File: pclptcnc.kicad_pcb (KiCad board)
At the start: 2 copper layers, 180.5 x 52.3 mm, 249 parts, among them P1 ARK825A-3, P3 ARK825A-4, P4 ARK825A-3, P5 ARK825A-3, P6 ARK825A-3, P7 ARK825A-3, P8 ARK825A-3, Q1 BC807-40, Q10 BC807-40, Q11 BC807-40, Q12 BC807-40, Q13 BC807-40, Q14 BC807-40, Q15 BC807-40, Q16 BC807-40, Q17 BC807-40, Q18 BC807-40, Q2 BC807-40, Q3 BC807-40, Q4 BC807-40, Q5 BC807-40, Q6 BC807-40, Q7 BC807-40, Q8 BC807-40, Q9 BC807-40, U1 74LVC1G3157GW, U10 SN74LVC2G17, U11 74HCT14, U12 SN74LVC2G17, U13 74HCT14, U2 HCPL2630, U3 HCPL2630, U4 HCPL2630, U5 HCPL2630, U6 HCPL2630, U7 HCPL2630, U8 74HCT14, U9 74HCT14, j1 DB25, j2 DB25

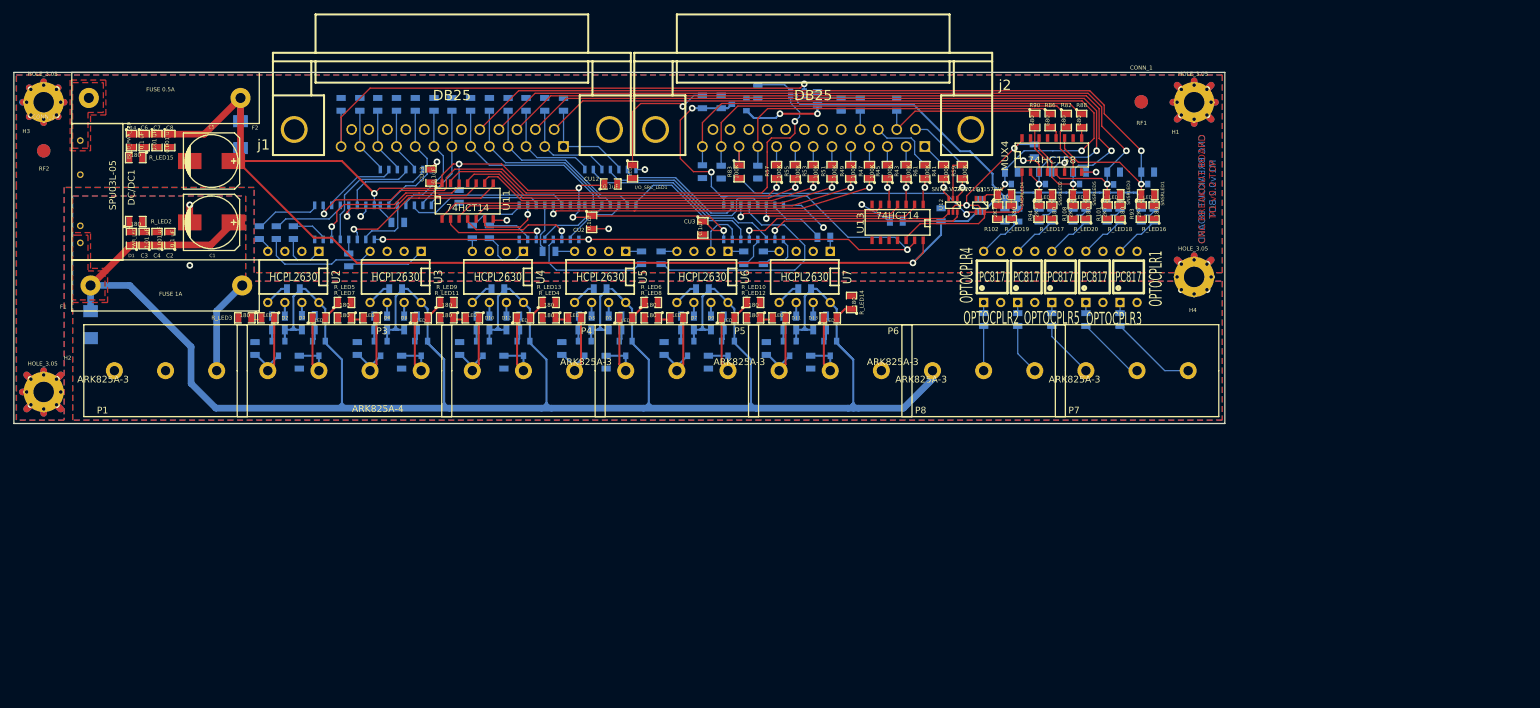
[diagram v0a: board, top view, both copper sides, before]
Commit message: revised first PCB version
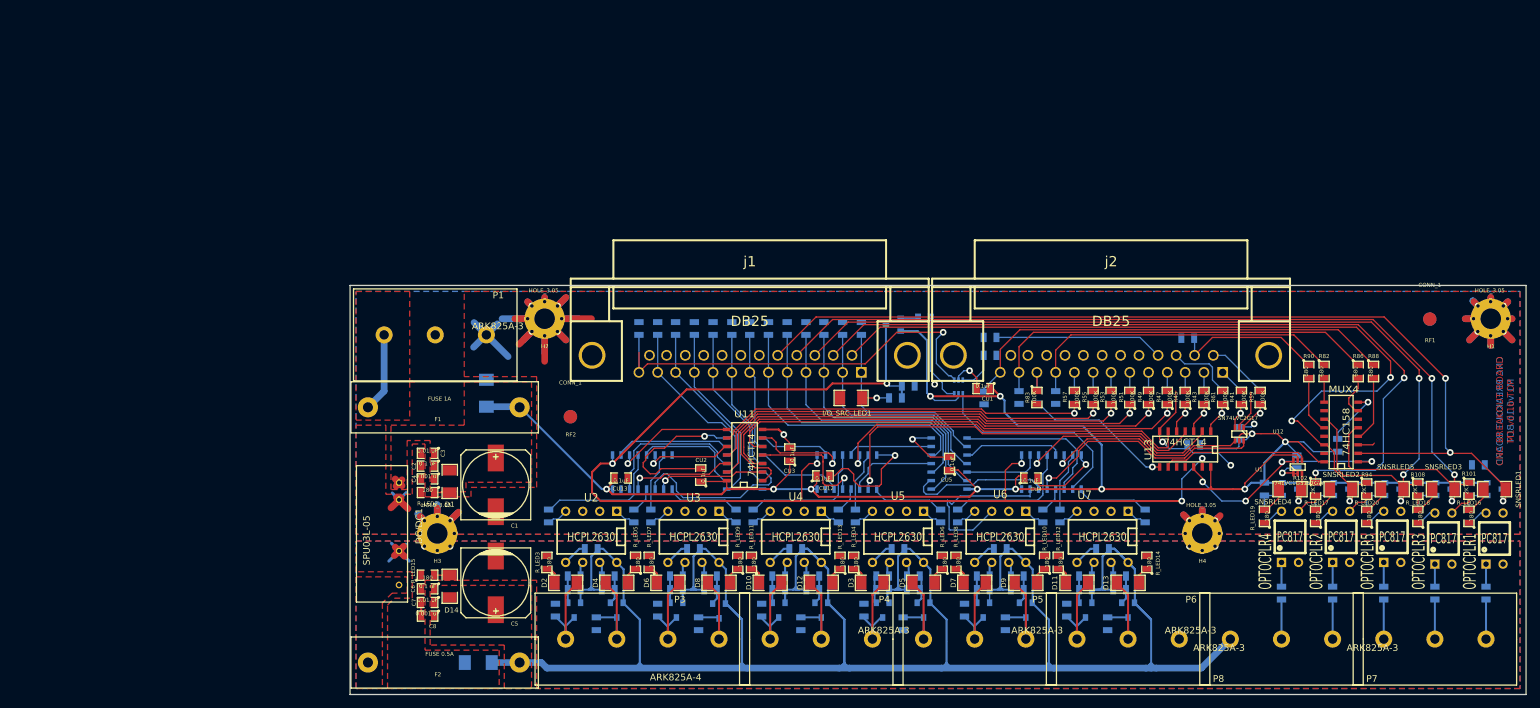
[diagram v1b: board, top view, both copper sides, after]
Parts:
- removed R123, R3, R4, R5, R6: 100K, SM0805
- C1, C5: footprint c_elec_8x10.5 -> c_elec_10x10
- CU1, CU4, CU5: moved to F.Cu
- D1, D10, D11, D12, D13, D14, D2, D3, D4, D5, D6, D7, D8, D9, I/O_SRC_LED1, SNSRLED1, SNSRLED2, SNSRLED3, SNSRLED4, SNSRLED5: footprint SM0805 -> SM1206
- Q1, Q10, Q11, Q12, Q13, Q14, Q15, Q16, Q17, Q18, Q2, Q3, Q4, Q5, Q6, Q7, Q8, Q9: footprint SOT23_ed -> SOT23
- R8: value 180 -> 2K7
- R93: moved to B.Cu
- moved CU15 121.5 mm to (211.8, 95.1), turned to 90 degrees
- moved F2 93.9 mm to (82.0, 129.2)
- moved CU1 90.7 mm to (173.7, 88.4), turned to 180 degrees
- moved RF2 87.9 mm to (112.2, 92.6) (x2)
- moved DC/DC1 87.1 mm to (87.9, 120.2), turned to 90 degrees
- moved H3 87.0 mm to (92.4, 110.0)
- moved TVS2 86.3 mm to (98.5, 129.2), turned to 0 degrees
- moved D14 81.6 mm to (94.2, 117.9), turned to 90 degrees
- moved C8 80.6 mm to (90.9, 122.3), turned to 180 degrees
- moved C7 79.8 mm to (90.9, 120.3), turned to 180 degrees
- moved C6 79.0 mm to (90.9, 118.2), turned to 180 degrees
- moved CU14 76.2 mm to (205.1, 96.8), turned to 180 degrees
- moved R_LED15 75.9 mm to (90.9, 116.2), turned to 0 degrees
- moved C5 75.8 mm to (101.1, 117.3), turned to 270 degrees
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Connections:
- net /RC_SW_INV renamed /PC/RC_SW_inv
- C1 pad 1: /ISOLATED_VCC -> VCC
- C1 pad 2: /ISOLATED_GND -> GND
- C2 pad 1: /ISOLATED_VCC -> VCC
- C2 pad 2: /ISOLATED_GND -> GND
- C3 pad 1: /ISOLATED_VCC -> VCC
- C3 pad 2: /ISOLATED_GND -> GND
- C4 pad 1: /ISOLATED_VCC -> VCC
- C4 pad 2: /ISOLATED_GND -> GND
- C5 pad 1: VCC -> /ISOLATED_VCC
- C5 pad 2: GND -> /ISOLATED_GND
- C6 pad 1: VCC -> /ISOLATED_VCC
- C6 pad 2: GND -> /ISOLATED_GND
- C7 pad 1: VCC -> /ISOLATED_VCC
- C7 pad 2: GND -> /ISOLATED_GND
- C8 pad 1: VCC -> /ISOLATED_VCC
- C8 pad 2: GND -> /ISOLATED_GND
- D1 pad 1: /ISOLATED_VCC -> VCC
- D14 pad 1: VCC -> /ISOLATED_VCC
- DC/DC1 pad 1: /ISOLATED_VCC -> VCC
- DC/DC1 pad 2: /ISOLATED_GND -> GND
- DC/DC1 pad 5: GND -> /ISOLATED_GND
- DC/DC1 pad 7: /VCC_NFused -> /ISOLATED_VCC_NFused
- F1 pad 1: /ISOLATED_VCC_NFused -> /VCC_NFused
- F1 pad 2: /ISOLATED_VCC -> VCC
- F2 pad 1: /VCC_NFused -> /ISOLATED_VCC_NFused
- F2 pad 2: VCC -> /ISOLATED_VCC
- MUX1 pad 11: /RC1 -> /RC4
- MUX1 pad 12: /FLTRD_SGNL3 -> /FLTRD_SGNL2
- MUX1 pad 13: /PC1 -> /PC3
- MUX1 pad 14: /RC2 -> /RC3
- MUX1 pad 2: /RC4 -> /RC2
- MUX1 pad 4: /FLTRD_SGNL4 -> /FLTRD_SGNL1
- MUX1 pad 5: /RC3 -> /RC1
- MUX1 pad 6: /PC3 -> /PC1
- MUX1 pad 7: /FLTRD_SGNL2 -> /FLTRD_SGNL3
- MUX1 pad 9: /FLTRD_SGNL1 -> /FLTRD_SGNL4
- MUX2 pad 10: /PC12 -> /PC8
- MUX2 pad 11: /RC7 -> /RC8
- MUX2 pad 12: /FLTRD_SGNL7 -> /FLTRD_SGNL6
- MUX2 pad 13: /PC5 -> /PC7
- MUX2 pad 14: /RC6 -> /RC7
- MUX2 pad 2: /RC11 -> /RC6
- MUX2 pad 3: /PC7 -> /PC6
- MUX2 pad 4: /FLTRD_SGNL8 -> /FLTRD_SGNL5
- MUX2 pad 5: /RC9 -> /RC5
- MUX2 pad 6: /PC6 -> /PC5
- MUX2 pad 7: /FLTRD_SGNL6 -> /FLTRD_SGNL7
- MUX2 pad 9: /FLTRD_SGNL5 -> /FLTRD_SGNL8
- MUX3 pad 10: /PC10 -> /PC12
- MUX3 pad 11: /RC10 -> /RC12
- MUX3 pad 13: /PC11 -> /PC10
- MUX3 pad 14: /RC12 -> /RC10
- MUX3 pad 2: /RC5 -> /RC9
- MUX3 pad 5: /RC8 -> /RC11
- MUX3 pad 6: /PC8 -> /PC11
- MUX3 pad 7: /FLTRD_SGNL12 -> /FLTRD_SGNL11
- MUX3 pad 9: /FLTRD_SGNL11 -> /FLTRD_SGNL12
- MUX4 pad 11: /SENSOR_1 -> /SENSOR_3
- MUX4 pad 12: /PC_IN_A3 -> /PC_IN_A5
- MUX4 pad 14: /SENSOR_3 -> /SENSOR_4
- MUX4 pad 2: /SENSOR_4 -> /SENSOR_1
- MUX4 pad 4: /PC_IN_A5 -> /PC_IN_A4
- MUX4 pad 7: /PC_IN_A1 -> /PC_IN_A3
- MUX4 pad 9: /PC_IN_A4 -> /PC_IN_A1
- P1 pad 1: /ISOLATED_VCC_NFused -> /VCC_NFused
- P1 pad 3: /ISOLATED_GND -> GND
- Q1 pad 1: /IOSRCTR_BASE -> N-0000096
- R111 pad 1: /SENSOR_1 -> /RCOUT2
- R112 pad 1: /SENSOR_2 -> /RCOUT3
- R113 pad 1: /SENSOR_3 -> /RCOUT4
- R114 pad 1: /SENSOR_4 -> /RCOUT5
- R115 pad 1: /SENSOR_5 -> /RCOUT6
- R116 pad 1: /RCOUT6 -> /RCOUT7
- R117 pad 1: /RCOUT7 -> /RCOUT8
- R118 pad 1: /RCOUT8 -> /RCOUT9
- R119 pad 1: /RCOUT9 -> /RCOUT10
- R120 pad 1: /RCOUT10 -> /RCOUT11
- R121 pad 1: /RCOUT11 -> /RCOUT12
- R122 pad 1: /RCOUT12 -> /SRC_SEL
- R2 pad 1: /CTRL_SRC -> N-0000096
- R2 pad 2: /IOSRCTR_BASE -> /CTRL_SRC
- R7 pad 1: /RCOUT5 -> /RCOUT1
- R_LED15 pad 1: GND -> /ISOLATED_GND
- R_LED2 pad 2: /ISOLATED_GND -> GND
- TVS1 pad 1: /ISOLATED_GND -> GND
- TVS1 pad 2: /ISOLATED_VCC -> VCC
- TVS2 pad 1: GND -> /ISOLATED_GND
- TVS2 pad 2: VCC -> /ISOLATED_VCC
- U1 pad 1: /SENSOR_5 -> GND
- U1 pad 3: GND -> /SENSOR_5
- U1 pad 4: /PC_IN_A2 -> /SNSR2
- U10 pad 4: /PC4 -> /PC12
- U11 pad 13: /PC_OUT_A9 -> /PC_OUT_A7
- U11 pad 2: /PC6 -> /PC4
- U11 pad 6: /PC12 -> /PC6
- U11 pad 9: /PC_OUT_A7 -> /PC_OUT_A9
- U13 pad 2: /PC8 -> /PC9
- U13 pad 4: /PC9 -> /PC8
- U13 pad 8: (no net) -> /PC_IN_A2
- U13 pad 9: (no net) -> /SNSR2
- U8 pad 1: /RCOUT3 -> /RCOUT4
- U8 pad 11: /RCOUT5 -> /RCOUT2
- U8 pad 13: /RCOUT6 -> /RCOUT3
- U8 pad 3: /RCOUT2 -> /RCOUT5
- U8 pad 5: /RCOUT1 -> /RCOUT6
- U8 pad 9: /RCOUT4 -> /RCOUT1
- U9 pad 1: /RCOUT12 -> /RCOUT10
- U9 pad 5: /RCOUT10 -> /RCOUT12
- j1 pad 14: /SENSOR_5 -> /SENSOR_4
- j1 pad 15: /SENSOR_4 -> /SENSOR_5
- j2 pad 10: /PC_IN3 -> /PC_IN1
- j2 pad 12: /PC_IN1 -> /PC_IN3
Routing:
- net /PC/RC_SW: track 144.8 -> 323.8 mm, vias 5 -> 6
- net GND: track 391.3 -> 531.7 mm, vias 42 -> 43
- net /ISOLATED_VCC: track 626.3 -> 542.3 mm
- net /PC4: track 90.5 -> 16.4 mm, vias 2 -> 1
- net VCC: track 395.6 -> 347.5 mm, vias 10 -> 11
- net /PC8: track 25.2 -> 58.6 mm
- net /SENSOR_2: track 120.2 -> 148.6 mm, vias 2 -> 3
- net /RCOUT3: track 15.7 -> 39.0 mm
- net /PC_OUT12: track 2.79 -> 25.2 mm
- net /SNSR2: track 0.00 -> 22.1 mm
- net /PC12: track 10.0 -> 31.5 mm, vias 1 -> 0
- net /SENSOR_1: track 130.0 -> 150.3 mm, vias 2 -> 3
- net /SENSOR_3: track 120.1 -> 139.7 mm, vias 2 -> 3
- net /RCOUT2: track 15.5 -> 34.3 mm
- net /RCOUT10: track 9.87 -> 26.9 mm
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- added copper zone on F.Cu, net /ISOLATED_VCC_NFused
- added copper zone on F.Cu, net VCC
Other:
- board size 180.5 x 52.3 mm -> 175.3 x 61 mm
- net class power added: clearance 0.15, trace_width 0.45, via_dia 1, via_drill 0.6
- rule pad_to_mask_clearance: 0 -> 0.05
- board text added: "CNC BREAKOUT BOARD M1 v0.1b BOT"
- board text added: "CNC BREAKOUT BOARD M1 v0.1b TOP"
- board text removed: "CNC BREAKOUT BOARD M1 v0.2 BOT"
- board text removed: "CNC BREAKOUT BOARD M1 v0.2 TOP"
